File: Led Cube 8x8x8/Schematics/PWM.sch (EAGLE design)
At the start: 6 parts, among them U1 TLC5941PWP

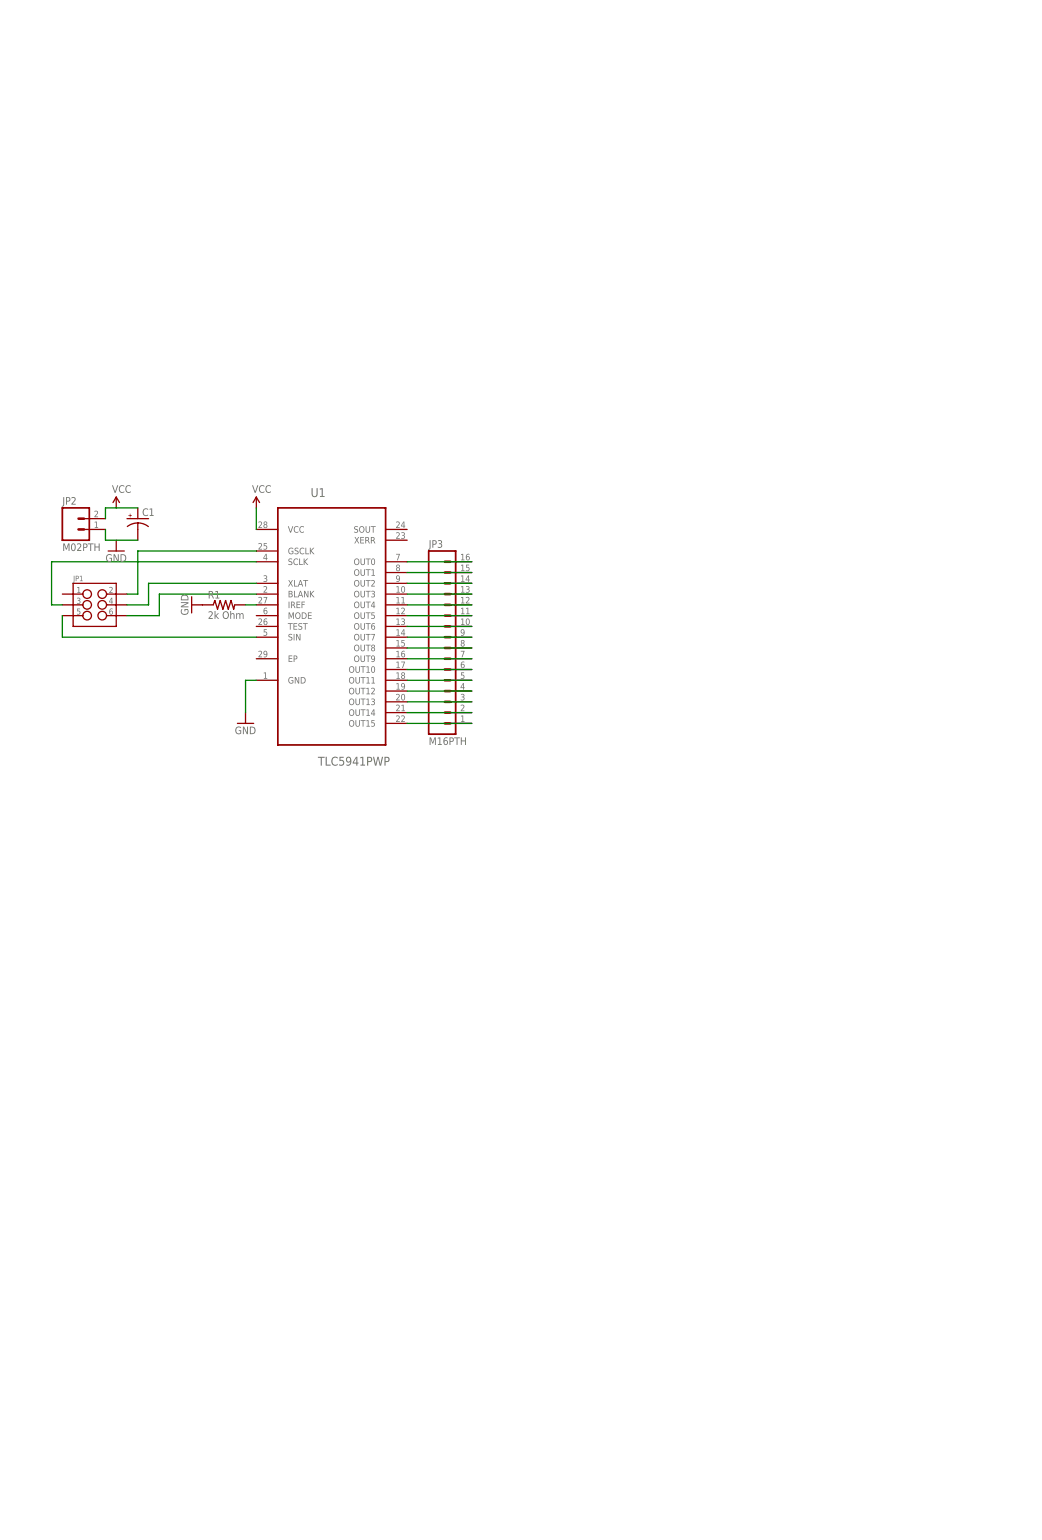
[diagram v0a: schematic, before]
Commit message: Updates
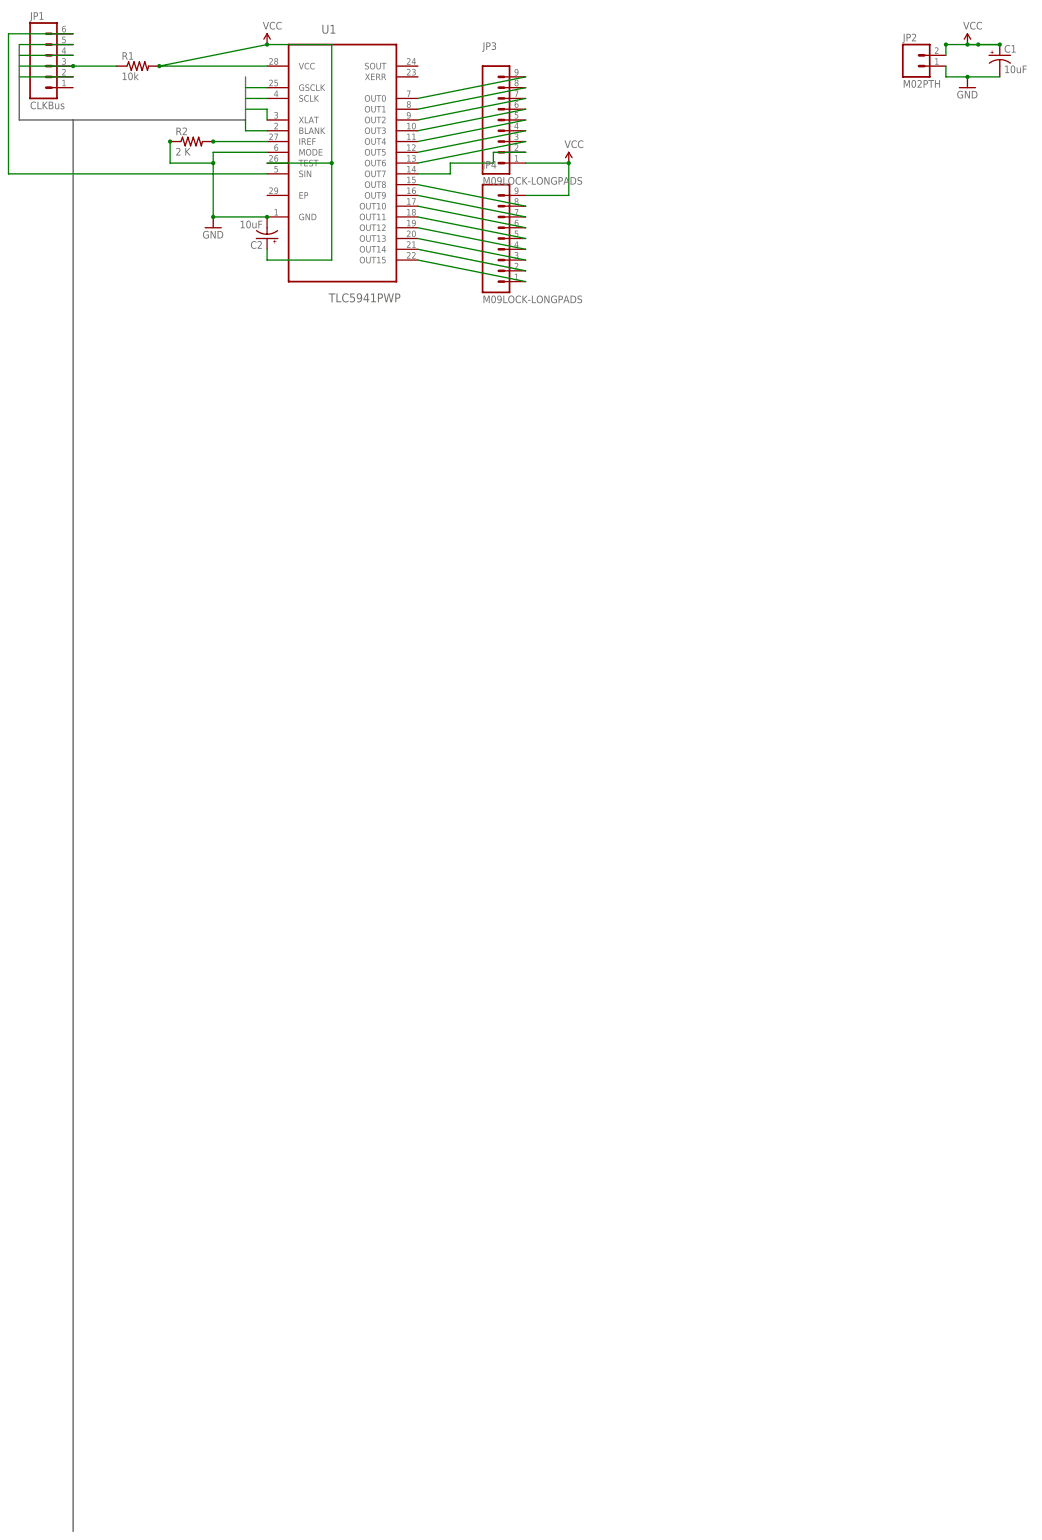
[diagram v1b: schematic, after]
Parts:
- added C2: 10uF, SparkFun-Capacitors:CAP_POLPTH2
- added JP4: M09LOCK-LONGPADS, SparkFun-Connectors:M09LOCK-LONGPADS
- added R2: 2 K, SparkFun-Resistors:RESISTORPTH-1/4W-VERT
- C1: value (none) -> 10uF
- JP1: value (none) -> CLKBus; device SparkFun-Connectors:M03X22X3_SILK_SM -> SparkFun-Connectors:M06LOCK_LONGPADS
- JP3: value M16PTH -> M09LOCK-LONGPADS; device SparkFun-Connectors:M16PTH -> SparkFun-Connectors:M09LOCK-LONGPADS
- R1: value 2k Ohm -> 10k; device SparkFun-Resistors:RESISTORPTH-1/4W -> SparkFun-Resistors:10KOHM-1/4W5%(PTH)VERT
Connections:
- net N$18 renamed GSCLK
- net N$19 renamed XLAT
- removed net N$17: JP3.1, U1.OUT15
- removed net N$20: JP1.6, U1.BLANK
- removed net N$21: JP1.5, U1.SIN
- removed net N$22: JP1.3, U1.SCLK
- removed net N$23: R1.2, U1.IREF
- new net BLANK: JP1.3, R1.1, U1.BLANK
- new net N$19: R2.2, U1.IREF
- new net SCLK: JP1.5, U1.SCLK
- new net SIN0: JP1.6, U1.SIN
- net GND: now also C1.-, C2.-, JP2.1, R2.1, U1.MODE; no longer R1.1
- net N$1: now also JP4.1, U1.OUT15; no longer C1.-, JP2.1
- net N$10: now also JP4.2, U1.OUT14; no longer JP3.8, U1.OUT8
- net N$11: now also JP4.3, U1.OUT13; no longer JP3.7, U1.OUT9
- net N$12: now also JP4.4, U1.OUT12; no longer JP3.6, U1.OUT10
- net N$13: now also JP4.5; no longer JP3.5
- net N$14: now also JP4.6, U1.OUT10; no longer JP3.4, U1.OUT12
- net N$15: now also JP4.7, U1.OUT9; no longer JP3.3, U1.OUT13
- net N$16: now also JP4.8, U1.OUT8; no longer JP3.2, U1.OUT14
- net N$2: now also JP3.2, U1.OUT7; no longer JP3.16, U1.OUT0
- net N$3: now also JP3.3, U1.OUT6; no longer JP3.15, U1.OUT1
- net N$4: now also JP3.4, U1.OUT5; no longer JP3.14, U1.OUT2
- net N$5: now also JP3.5, U1.OUT4; no longer JP3.13, U1.OUT3
- net N$6: now also JP3.6, U1.OUT3; no longer JP3.12, U1.OUT4
- net N$7: now also JP3.7, U1.OUT2; no longer JP3.11, U1.OUT5
- net N$8: now also JP3.8, U1.OUT1; no longer JP3.10, U1.OUT6
- net N$9: now also U1.OUT0; no longer U1.OUT7
- net VCC: now also C2.+, JP3.1, JP4.9, R1.2, U1.TEST
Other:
- moved on the sheet: C1, JP2, R1, U1

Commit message: FRMR
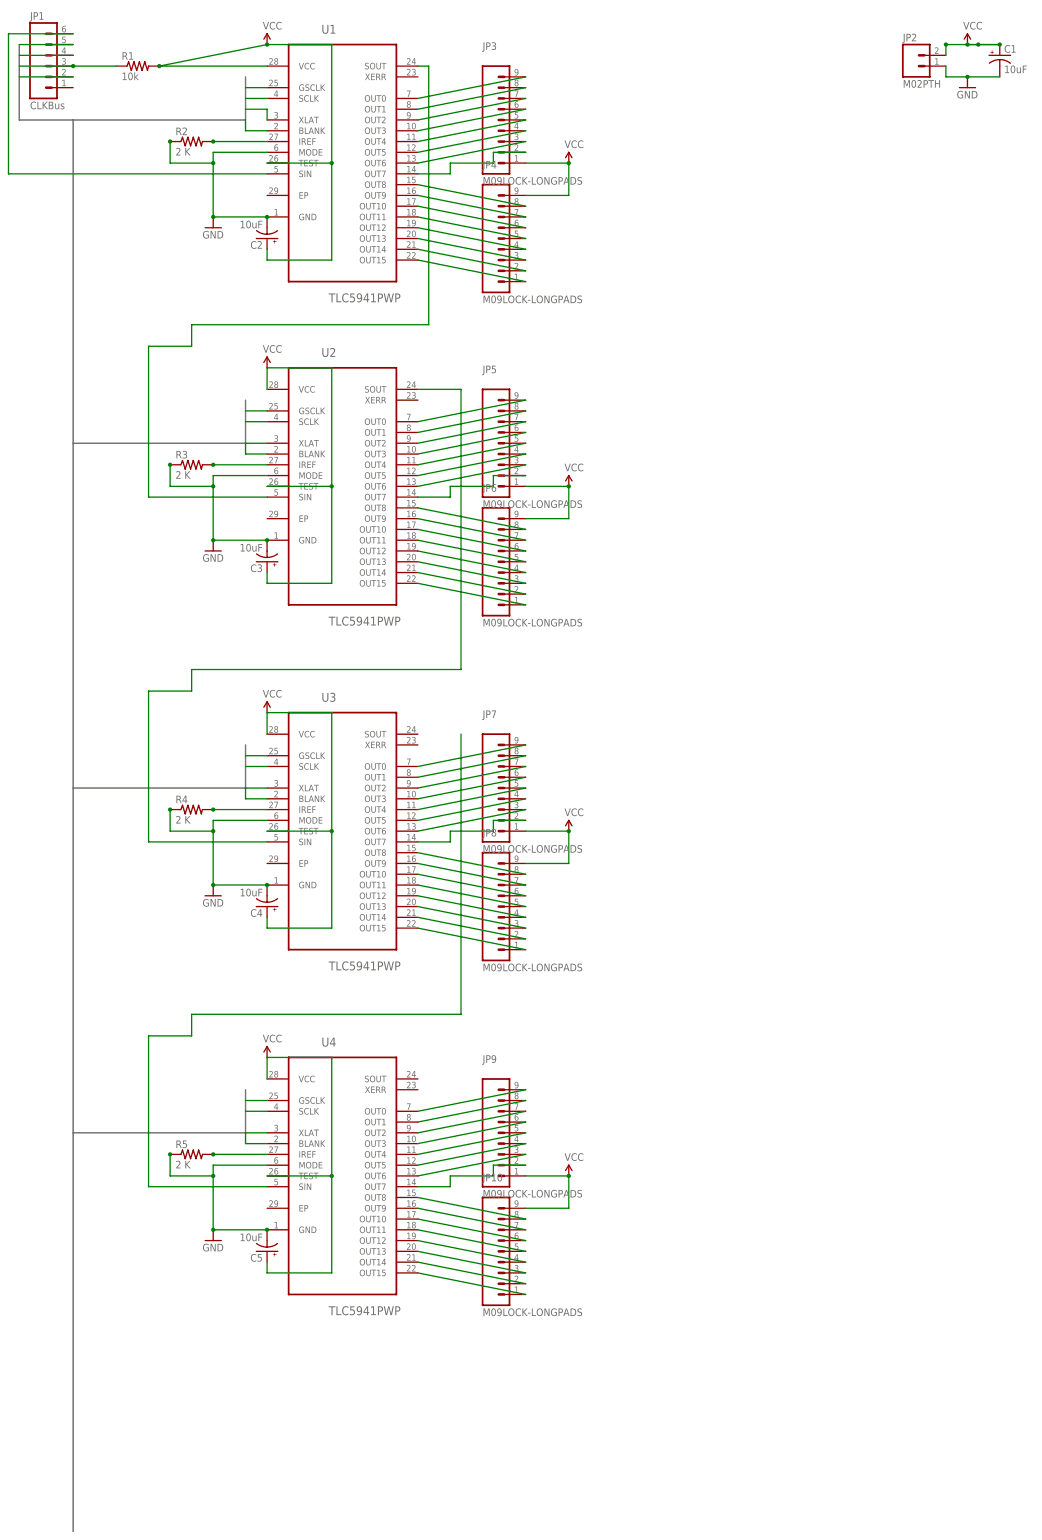
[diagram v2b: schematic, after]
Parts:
- added C3, C4, C5: 10uF, SparkFun-Capacitors:CAP_POLPTH2
- added JP10, JP5, JP6, JP7, JP8, JP9: M09LOCK-LONGPADS, SparkFun-Connectors:M09LOCK-LONGPADS
- added R3, R4, R5: 2 K, SparkFun-Resistors:1KOHM1/4W5%(PTH)
- added U2, U3, U4: TLC5941PWP, Texas Instruments_By_element14_Batch_1:TLC5941PWP
- R1: device SparkFun-Resistors:10KOHM-1/4W5%(PTH)VERT -> SparkFun-Resistors:10KOHM-1/4W-1%(PTH)HORIZ
- R2: device SparkFun-Resistors:RESISTORPTH-1/4W-VERT -> SparkFun-Resistors:1KOHM1/4W5%(PTH)
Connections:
- new net N$24: R3.2, U2.IREF
- new net N$25: JP5.3, U2.OUT6
- new net N$26: JP5.4, U2.OUT5
- new net N$27: JP5.5, U2.OUT4
- new net N$28: JP5.6, U2.OUT3
- new net N$29: JP5.7, U2.OUT2
- new net N$30: JP5.8, U2.OUT1
- new net N$31: JP5.9, U2.OUT0
- new net N$32: JP6.1, U2.OUT15
- new net N$33: JP6.2, U2.OUT14
- new net N$34: JP6.3, U2.OUT13
- new net N$35: JP6.4, U2.OUT12
- new net N$36: JP6.5, U2.OUT11
- new net N$37: JP6.6, U2.OUT10
- new net N$38: JP6.7, U2.OUT9
- new net N$39: JP6.8, U2.OUT8
- new net N$40: JP5.2, U2.OUT7
- new net N$44: R4.2, U3.IREF
- new net N$46: JP7.3, U3.OUT6
- new net N$47: JP7.4, U3.OUT5
- new net N$48: JP7.5, U3.OUT4
- new net N$49: JP7.6, U3.OUT3
- new net N$50: JP7.7, U3.OUT2
- new net N$51: JP7.8, U3.OUT1
- new net N$52: JP7.9, U3.OUT0
- new net N$53: JP8.1, U3.OUT15
- new net N$54: JP8.2, U3.OUT14
- new net N$55: JP8.3, U3.OUT13
- new net N$56: JP8.4, U3.OUT12
- new net N$57: JP8.5, U3.OUT11
- new net N$58: JP8.6, U3.OUT10
- new net N$59: JP8.7, U3.OUT9
- new net N$60: JP8.8, U3.OUT8
- new net N$61: JP7.2, U3.OUT7
- new net N$62: R5.2, U4.IREF
- new net N$63: JP9.3, U4.OUT6
- new net N$64: JP9.4, U4.OUT5
- new net N$65: JP9.5, U4.OUT4
- new net N$66: JP9.6, U4.OUT3
- new net N$67: JP9.7, U4.OUT2
- new net N$68: JP9.8, U4.OUT1
- new net N$69: JP9.9, U4.OUT0
- new net N$70: JP10.1, U4.OUT15
- new net N$71: JP10.2, U4.OUT14
- new net N$72: JP10.3, U4.OUT13
- new net N$73: JP10.4, U4.OUT12
- new net N$74: JP10.5, U4.OUT11
- new net N$75: JP10.6, U4.OUT10
- new net N$76: JP10.7, U4.OUT9
- new net N$77: JP10.8, U4.OUT8
- new net N$78: JP9.2, U4.OUT7
- new net SIN1: U1.SOUT, U2.SIN
- new net SIN2: U2.SOUT, U3.SIN
- new net SIN3: U4.SIN
- net BLANK: now also U2.BLANK, U3.BLANK, U4.BLANK
- net GND: now also C3.-, C4.-, C5.-, R3.1, R4.1, R5.1, U2.GND, U2.MODE, U3.GND, U3.MODE, U4.GND, U4.MODE
- net GSCLK: now also U2.GSCLK, U3.GSCLK, U4.GSCLK
- net SCLK: now also U2.SCLK, U3.SCLK, U4.SCLK
- net VCC: now also C3.+, C4.+, C5.+, JP10.9, JP5.1, JP6.9, JP7.1, JP8.9, JP9.1, U2.TEST, U2.VCC, U3.TEST, U3.VCC, U4.TEST, U4.VCC
- net XLAT: now also U2.XLAT, U3.XLAT, U4.XLAT
